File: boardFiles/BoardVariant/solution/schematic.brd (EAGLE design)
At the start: 88.6 x 63.5 mm, 4 parts, among them IC1 MSP430F1491, IC2 BQ24120

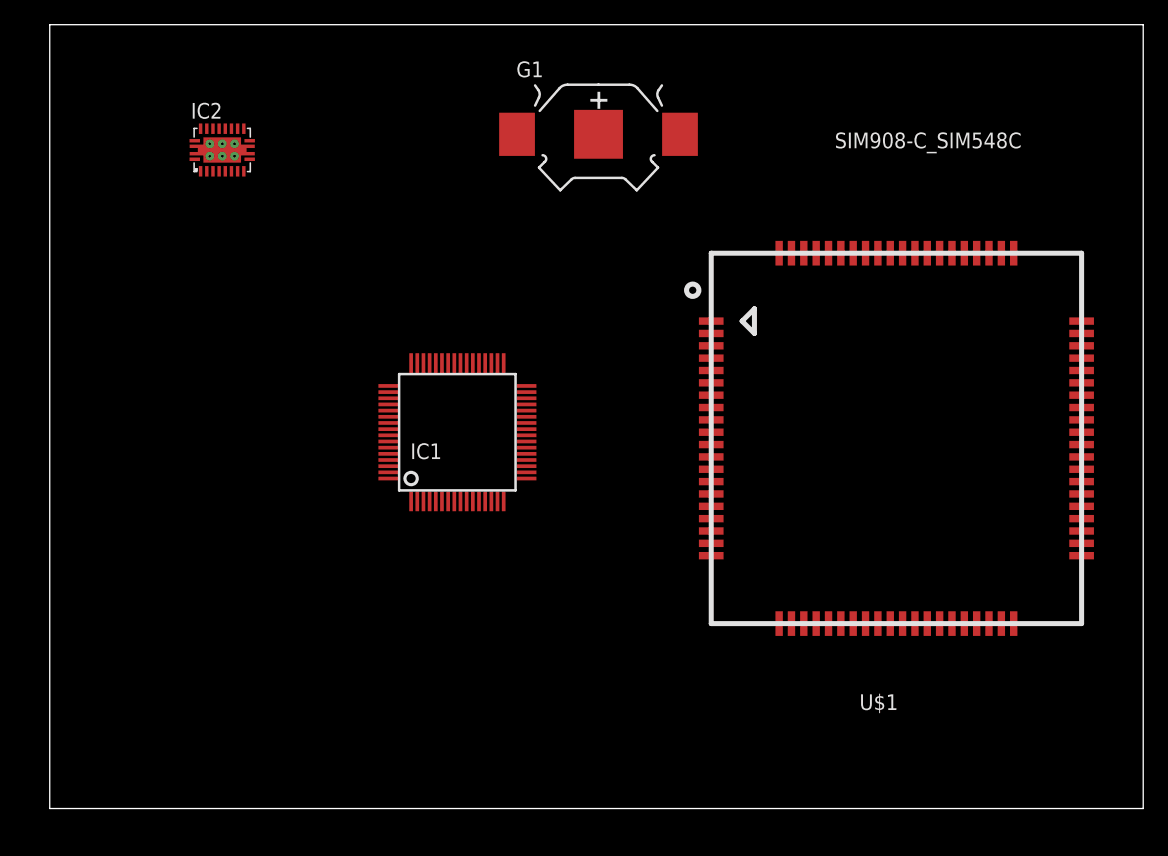
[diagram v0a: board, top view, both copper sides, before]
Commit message: Normal Push.
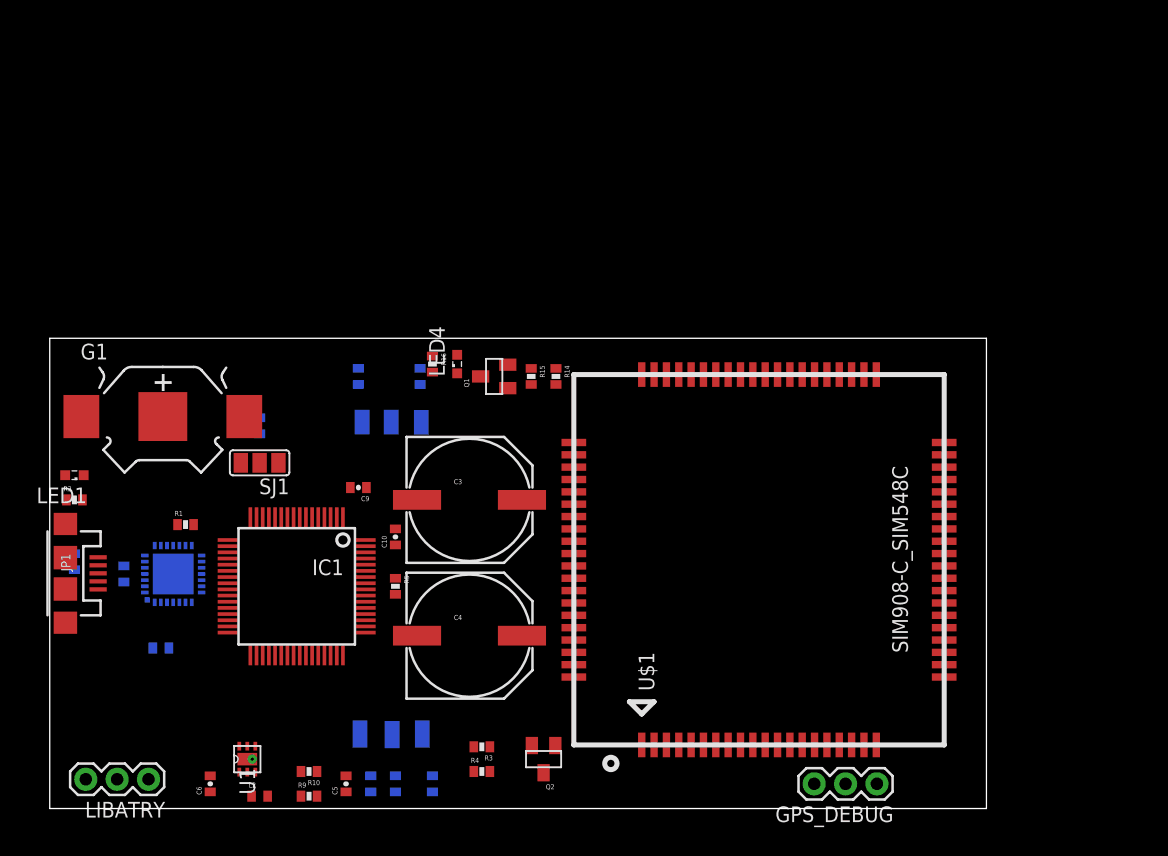
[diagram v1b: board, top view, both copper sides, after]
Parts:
- removed IC2: BQ24120, texas:QFN20_3,5X4,5
- added C1, C10, C11, C12, C2, C9: 10uF, SparkFun-Capacitors:0402-CAP
- added C3, C4: 400uF, SparkFun-Capacitors:PANASONIC_G
- added C5: 22pF, SparkFun-Capacitors:0402-CAP
- added C6: 4.7uF, SparkFun-Capacitors:0402-CAP
- added C7, C8: 100nF, SparkFun-Capacitors:0402-CAP
- added GPS_DEBUG, LIBATRY: (no value), SparkFun-Connectors:1X03
- added IC3: CP2102, silabs:MLP28
- added JP1: USB-MICROB, SparkFun-Connectors:USB-MICROB
- added L2: 22uH, SparkFun-Passives:C0402
- added LED1, LED4: (no value), led:SML0603
- added Q1, Q2: (no value), SparkFun-DiscreteSemi:SOT23
- added R1: 0R, SparkFun-Passives:0402-RES
- added R10: 240k, SparkFun:0402-RES
- added R11, R12, R13: 22R, SparkFun:0402-RES
- added R14, R15: (no value), SparkFun-Passives:0402-RES
- added R16: (no value), SparkFun:0402-RES
- added R2, R5: 470, SparkFun-Passives:0402-RES
- added R3: 4.7k, SparkFun-Passives:0402-RES
- added R4: 47k, SparkFun-Passives:0402-RES
- added R9: 300k, SparkFun:0402-RES
- added SJ1: (no value), jumper:SJ_2
- added U$2: SIMHOLDER3, SparkFun-Connectors:SIMHOLDER3
- added U1: TPS62122_DRV_6, myTracelib:DRV6_1P6X1
- moved G1 42.0 mm to (9.16, 31.8)
- moved IC1 18.0 mm to (20.0, 18.0), turned to 180 degrees
- moved U$1 15.6 mm to (57.0, 20.1), turned to 90 degrees
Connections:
- removed net AVCC: IC1.64
- removed net AVSS: IC1.62
- removed net DVCC: IC1.1
- removed net DVSS: IC1.63
- removed net VSS: IC2.10
- new net GND: C1.1, C10.1, C11.1, C2.1, C3.-, C4.-, C6.2, C7.1, C8.1, C9.1, G1.-, GPS_DEBUG.1, IC1.11, IC1.62, IC1.63, IC3.3, IC3.EXP, IC3.M, JP1.GND, JP1.MT1, JP1.MT2, LED1.C, LIBATRY.3, Q2.2, R10.1, R4.1, U$1.P$1, U$1.P$10, U$1.P$14, U$1.P$2, U$1.P$37, U$1.P$40, U$1.P$41, U$1.P$43, U$1.P$5, U$1.P$57, U$1.P$58, U$1.P$60, U$1.P$61, U$1.P$64, U$1.P$65, U$1.P$77, U$1.P$78, U$1.P$80, U$2.6, U1.6
- new net GPS_RXD: GPS_DEBUG.2, U$1.P$16
- new net GPS_TXD: GPS_DEBUG.3, U$1.P$15
- new net GSM_CTS: IC1.13, U$1.P$67
- new net GSM_DCD: IC1.14, U$1.P$70
- new net GSM_DTR: IC1.16, U$1.P$72
- new net GSM_PWRKEY: IC1.18, R3.2
- new net GSM_RI: IC1.15, U$1.P$69
- new net GSM_RTS: IC1.12, U$1.P$66
- new net GSM_STATUS: IC1.17, U$1.P$52
- new net N$10: R11.1, U$2.2
- new net N$11: C2.2, IC3.6
- new net N$12: L2.1, U1.1
- new net N$14: C11.2, SJ1.2
- new net N$15: IC3.7, IC3.8, IC3.9, R1.2, R2.2
- new net N$16: R12.1, U$2.3
- new net N$17: R13.2, U$2.4
- new net N$19: C5.2, R10.2, R9.1, U1.3
- new net N$2: IC1.7, SJ1.1
- new net N$21: C12.2, IC3.28
- new net N$23: Q1.2, R15.1
- new net N$24: Q1.1, R14.2, R15.2
- new net N$25: IC1.19
- new net N$4: LED4.C, Q1.3
- new net N$5: LED1.A, R2.1
- new net N$7: LED4.A, R16.1
- new net N$8: Q2.1, R3.1, R4.2
- new net NETL: R14.1, U$1.P$51
- new net NTC: LIBATRY.2, U$1.P$73
- new net PWRKEY: Q2.3, U$1.P$3
- new net RESET: C12.1, IC1.58, R5.1
- new net SIM_CLK: R12.2, U$1.P$19
- new net SIM_DATA: C8.2, R13.1, U$1.P$17
- new net SIM_RST: R11.2, U$1.P$18
- new net SIM_VDD: C7.2, U$1.P$20, U$2.1
- new net UART0_RXD: IC1.33, IC3.26
- new net UART0_TXD: IC1.32, IC3.25
- new net UART1_RXD: IC1.35, U$1.P$71
- new net UART1_TXD: IC1.34, U$1.P$68
- new net USB_N: IC3.5, JP1.D-
- new net USB_P: IC3.4, JP1.D+
- new net VBAT: C3.+, C4.+, LIBATRY.1, R16.2, U$1.P$62, U$1.P$63, U1.4, U1.5
- new net VBUS: C1.2, JP1.VBUS, R1.1, U$1.P$74
- new net VDD: C10.2, C5.1, C6.1, C9.2, IC1.1, IC1.10, IC1.64, L2.2, R5.2, R9.2, U1.2
- new net VRTC: G1.+@1, G1.+@2, U$1.P$42
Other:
- board size 88.6 x 63.5 mm -> 75.9 x 38.1 mm
